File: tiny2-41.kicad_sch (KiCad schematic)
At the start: 22 parts, among them J1 Conn_01x01_Male, J10 Conn_01x01_Male, J11 Conn_01x01_Male, J12 Conn_01x01_Male, J2 Conn_01x01_Male, J20 Conn_01x04_Female, J21 Conn_01x08_Male, J3 Conn_01x01_Male, J4 Conn_01x01_Male, J5 Conn_01x01_Male, J6 Conn_01x01_Male, J7 Conn_01x01_Male, J8 Conn_01x01_Male, J9 Conn_01x01_Male, U1 4050, U2 CD40109BE, U3 Pico, U4 MB85RS1MT

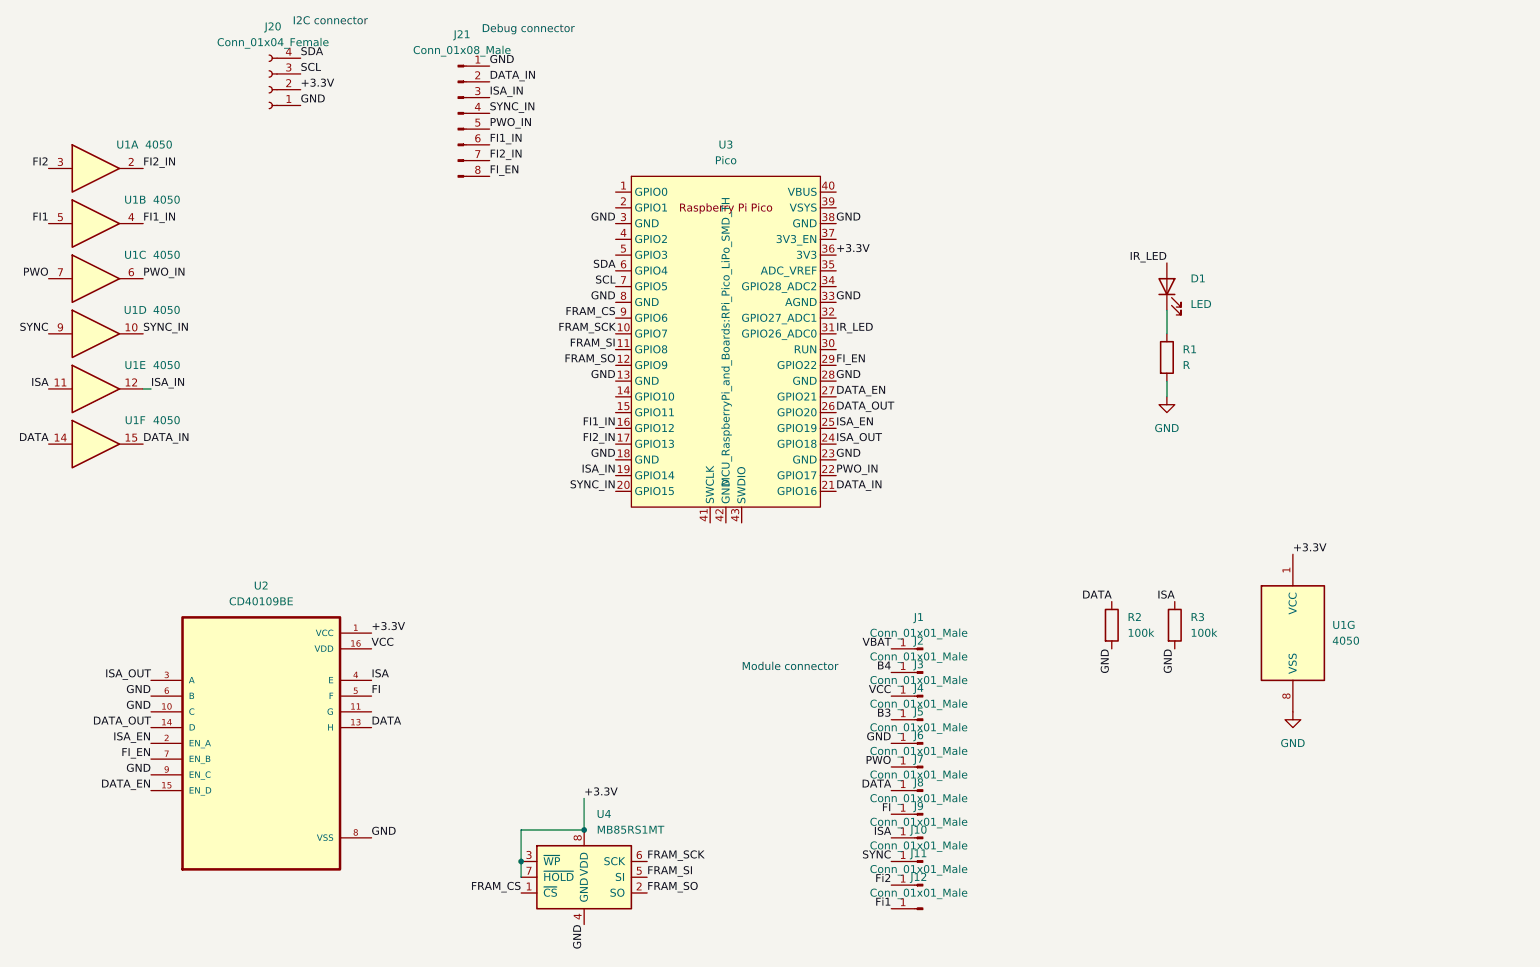
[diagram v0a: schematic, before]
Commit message: Updated ...
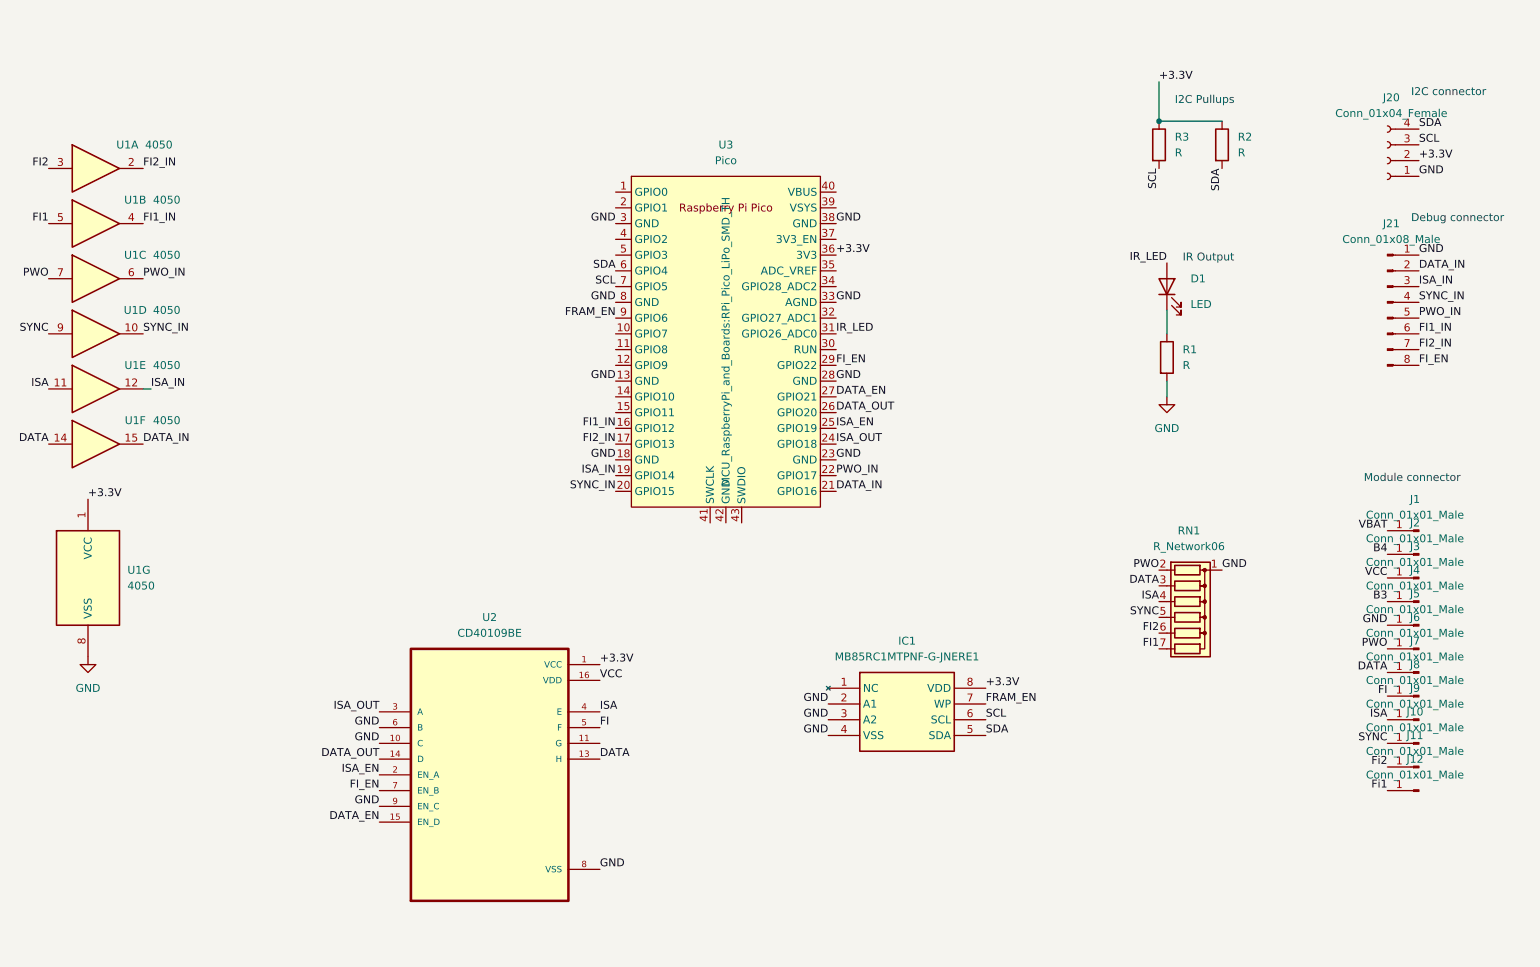
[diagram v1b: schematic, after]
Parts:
- removed U4: MB85RS1MT, symbol Memory_NVRAM:MB85RS1MT
- added IC1: MB85RC1MTPNF-G-JNERE1, KiCad:SOIC127P600X175-8N, symbol MB85RC1MTPNF-G-JNERE1:MB85RC1MTPNF-G-JNERE1
- added RN1: R_Network06, KiCad:4607X101105LF, symbol Device:R_Network06
- R2, R3: value 100k -> R
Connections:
- net +3.3V: now also R2.1, R3.1, IC1.8 (VDD)
- net DATA: now also RN1.3 (R2); no longer R2.1
- net FI1: now also RN1.7 (R6)
- net FI2: now also RN1.6 (R5)
- net GND: now also IC1.2 (A1), IC1.3 (A2), IC1.4 (VSS), RN1.1 (common); no longer R2.2, R3.2
- net ISA: now also RN1.4 (R3); no longer R3.1
- net PWO: now also RN1.2 (R1)
- net SCL: now also R3.2, IC1.6 (SCL)
- net SDA: now also R2.2, IC1.5 (SDA)
- net SYNC: now also RN1.5 (R4)
- net FRAM_CS renamed FRAM_EN
- net FRAM_EN: now also IC1.7 (WP)
- net FRAM_SCK: no longer names the net of U3.10 (GPIO7)
- net FRAM_SI: no longer names the net of U3.11 (GPIO8)
- net FRAM_SO: no longer names the net of U3.12 (GPIO9)
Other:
- note added: "I2C Pullups"
- note added: "IR Output"
- moved on the sheet: J1, J10, J11, J12, J2, J20, J21, J3, J4, J5, J6, J7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
